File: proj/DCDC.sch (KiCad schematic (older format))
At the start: 48 parts, among them Q13 MMBT3904, Q15 MMBT3904, Q16 MMBT3904, Q17 PZT2907A, Q18 PZT2907A, Q19 MMBT3904, U14 L78M05CDT, U15 MC79M05CDT, U16 AZ1117CH-1.8TRG1, U17 MCP1700T-vv02E/TT

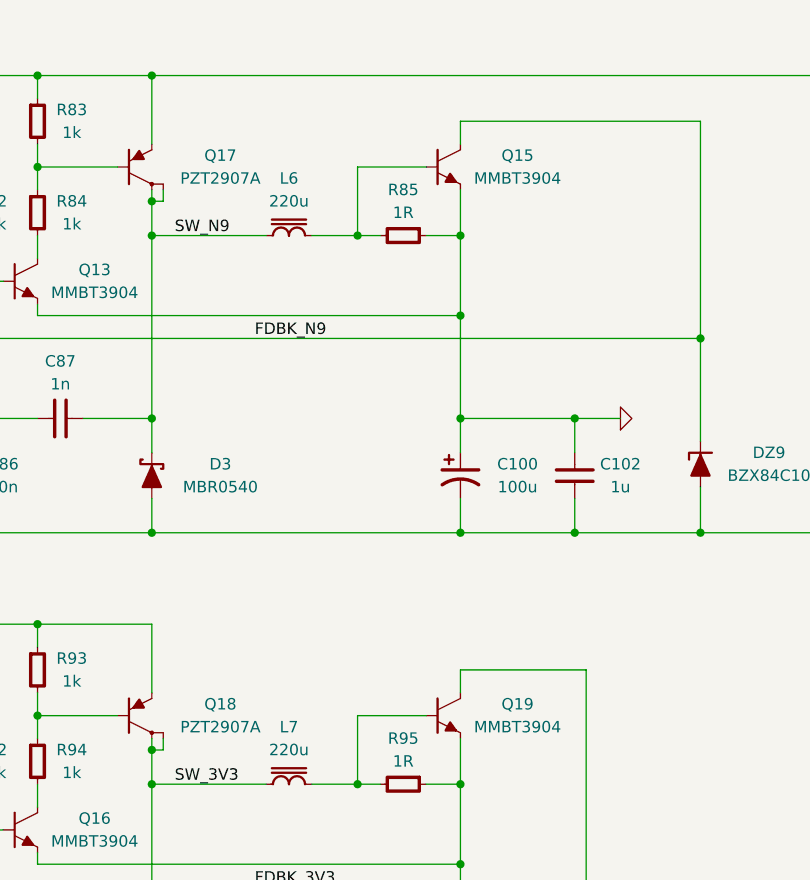
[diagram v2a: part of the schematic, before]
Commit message: Lots of routing
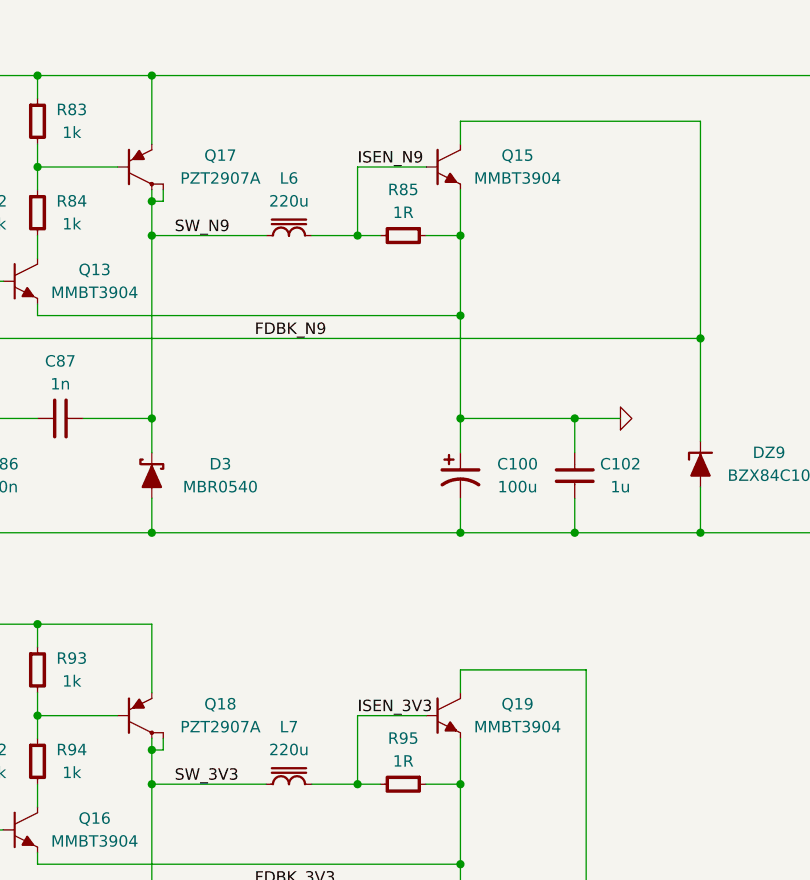
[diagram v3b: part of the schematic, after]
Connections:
- net ISEN_N9: now reaches L6.1, Q15.1, R85.2
- net ISEN_3V3: now reaches L7.1, Q19.1, R95.2
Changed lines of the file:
@@
 Wire Wire Line
 	4300 2900 10600 2900
+Text Label 6050 1300 0    50   ~ 0
+ISEN_N9
+Text Label 6050 3700 0    50   ~ 0
+ISEN_3V3
 $EndSCHEMATC
